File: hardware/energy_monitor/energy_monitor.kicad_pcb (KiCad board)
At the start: 2 copper layers, 102.8 x 86.9 mm, 137 parts, among them J1 Screw_Terminal_01x03, J2 SJ1-3533NG, J3 SJ1-3533NG, J4 SJ1-3533NG, J5 SJ1-3533NG, J6 SJ1-3533NG, J7 SJ1-3533NG, J8 USB_OTG, Q1 MMBT2222, Q2 MMBT2222, U1 RAC04, U2 TPS730, U3 TPS723, U4 ADS131E08, U5 AP2112, U6 ESP-WROOM-32U, U7 CP2104

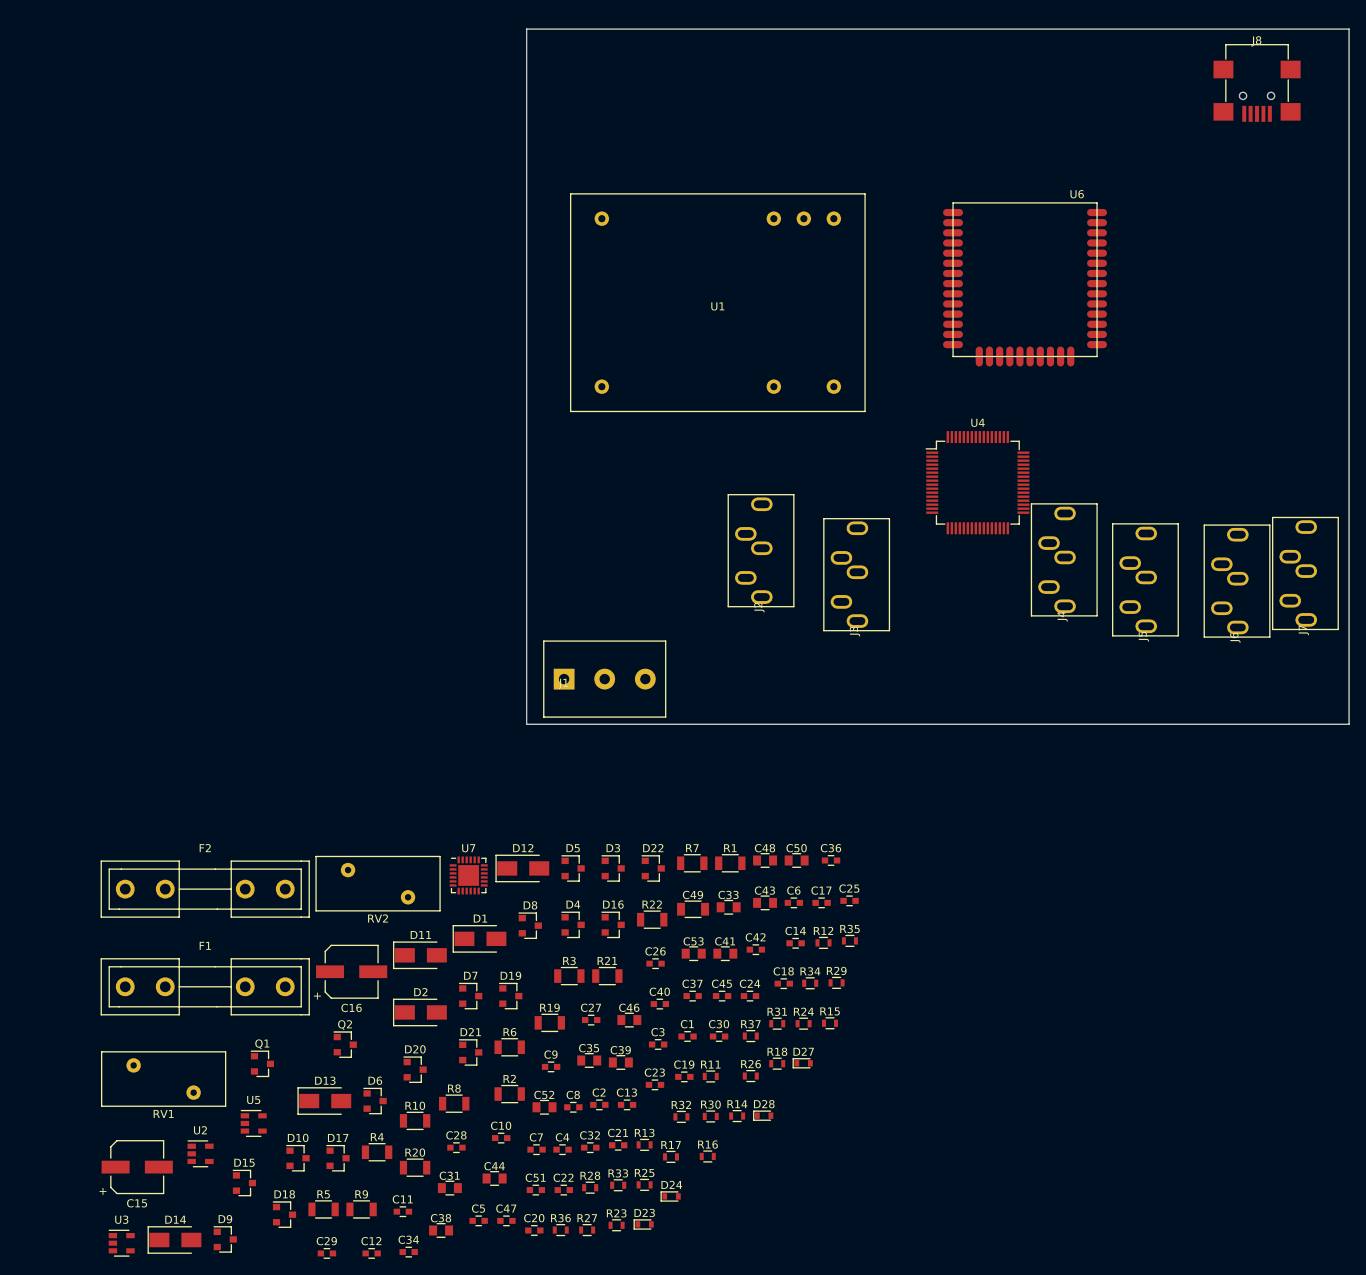
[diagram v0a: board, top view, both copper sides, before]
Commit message: Working on layout
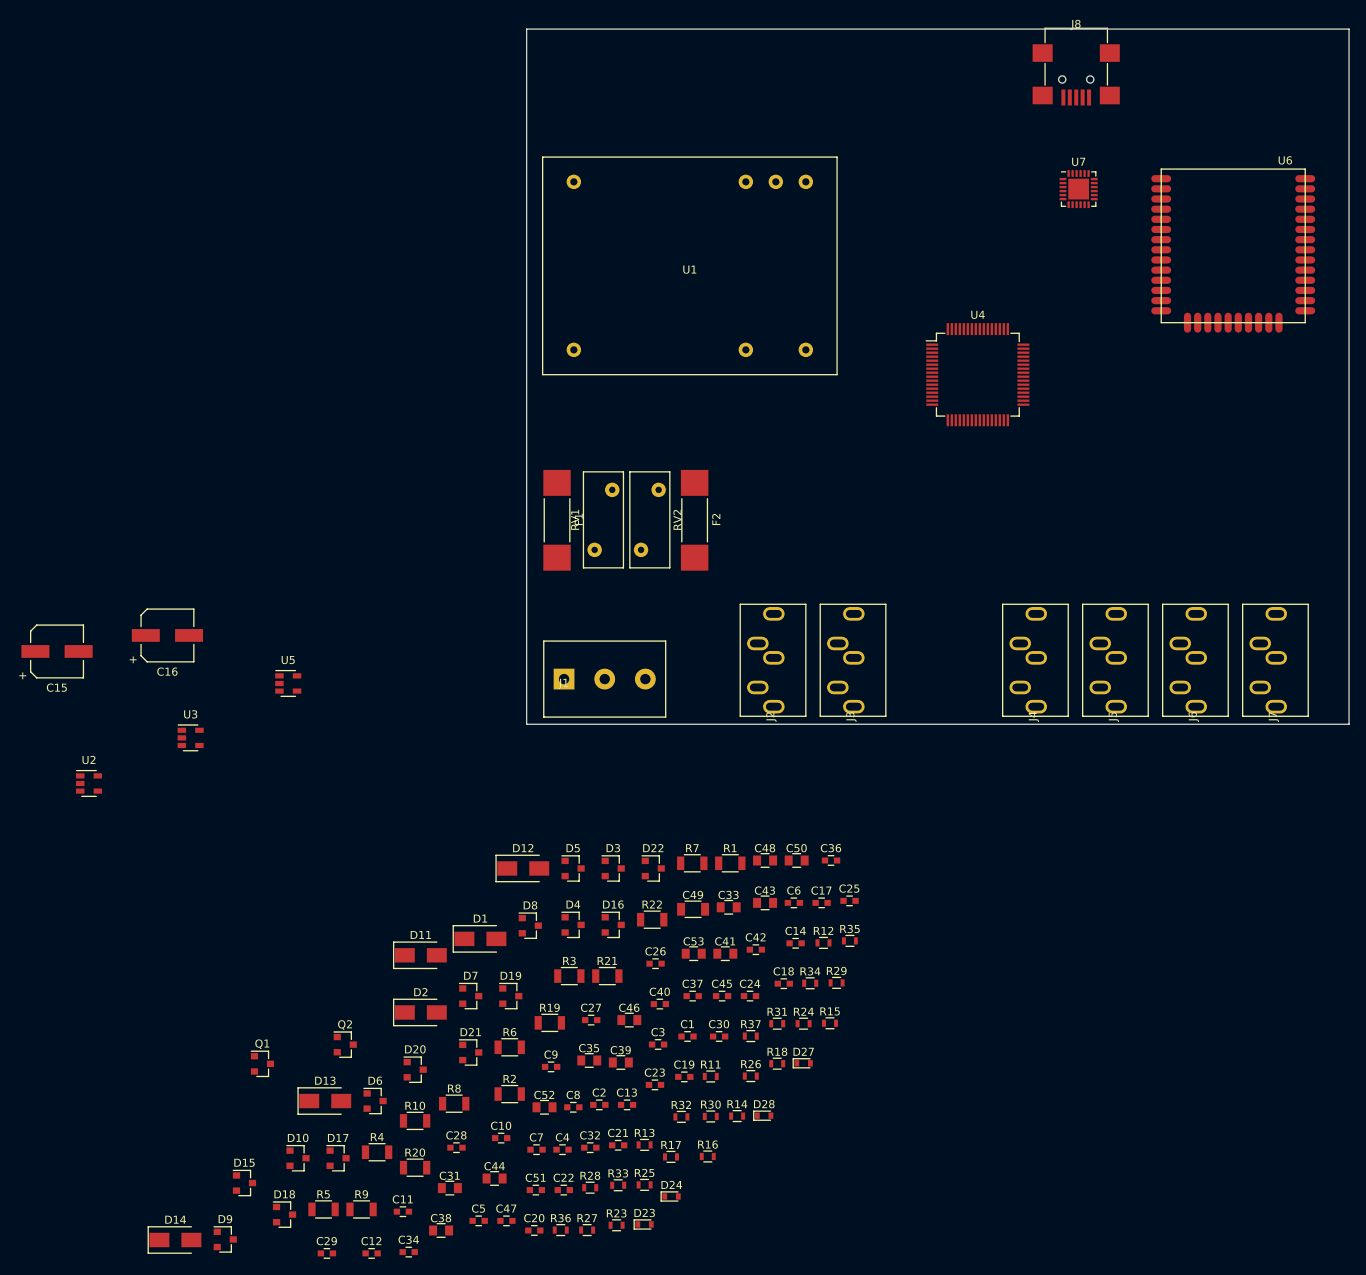
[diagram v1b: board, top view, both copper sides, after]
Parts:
- F1, F2: footprint Fuse_Holders_and_Fuses:Fuseholder5x20_horiz_open_inline_Type-I -> footprint:Fuse_Littelfuse-443
- RV1, RV2: footprint Varistors:RV_Disc_D15.5_W6.8_P7.5 -> Varistors:RV_Disc_D12_W5_P7.5
- moved U7 114.8 mm to (159.0, 53.1)
- moved RV1 93.6 mm to (100.7, 90.7), turned to 270 degrees
- moved F2 84.8 mm to (111.0, 94.5), turned to 270 degrees
- moved F1 79.5 mm to (93.8, 94.5), turned to 270 degrees
- moved C15 65.2 mm to (31.3, 110.9)
- moved U3 63.7 mm to (48.0, 121.7)
- moved U5 55.2 mm to (60.2, 114.9)
- moved RV2 54.3 mm to (104.3, 98.2), turned to 90 degrees
- moved U2 48.3 mm to (35.3, 127.4)
- moved C16 47.9 mm to (45.1, 108.9)
- moved U6 26.4 mm to (178.3, 57.0)
- moved J8 22.7 mm to (158.7, 33.0)
- moved J2 13.8 mm to (120.0, 119.0)
- moved U4 13.5 mm to (146.4, 76.3)
- moved J4 13.1 mm to (152.8, 119.0)
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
